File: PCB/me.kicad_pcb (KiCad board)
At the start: 2 copper layers, 166.7 x 154.5 mm, 14 parts, among them M1 Motor_DC, Q1 AO3400A, SW1 SW_Push, SW2 SW_Push, SW3 SW_Push, SW4 SW_Push, SW5 SW_Push, SW6 SW_Push, U1 XIAO-RP2040-DIP

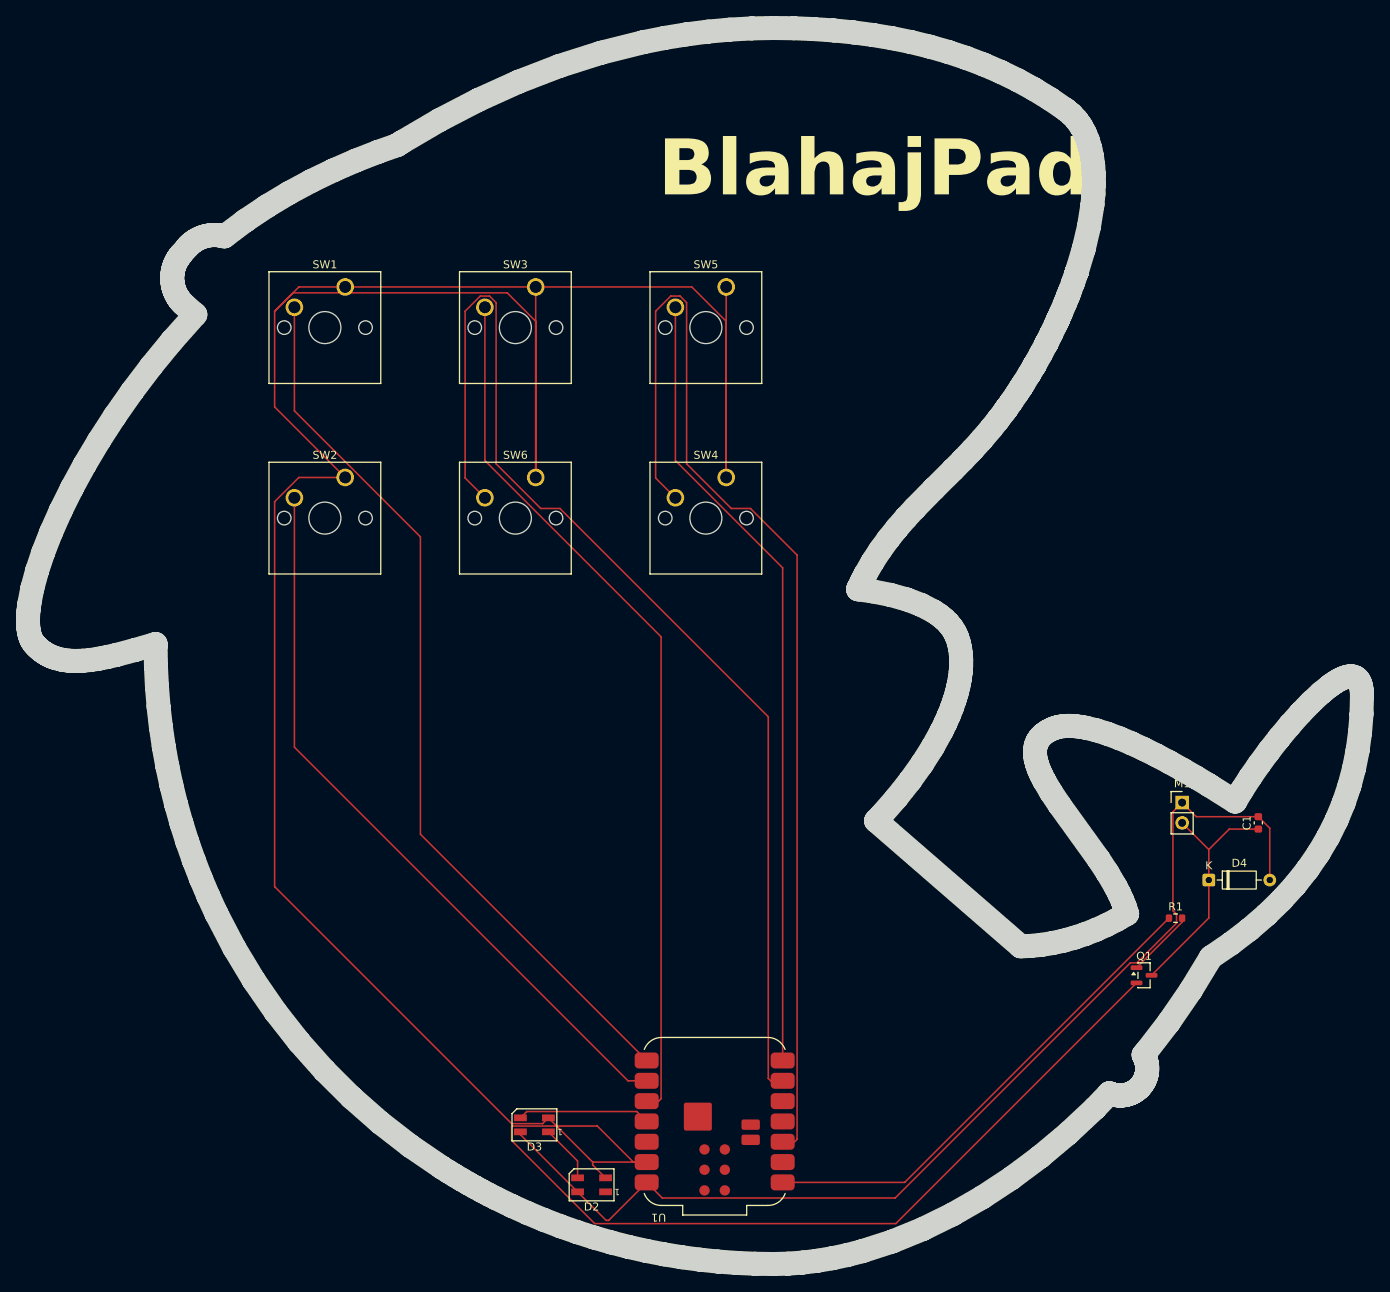
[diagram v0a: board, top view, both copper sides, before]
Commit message: please
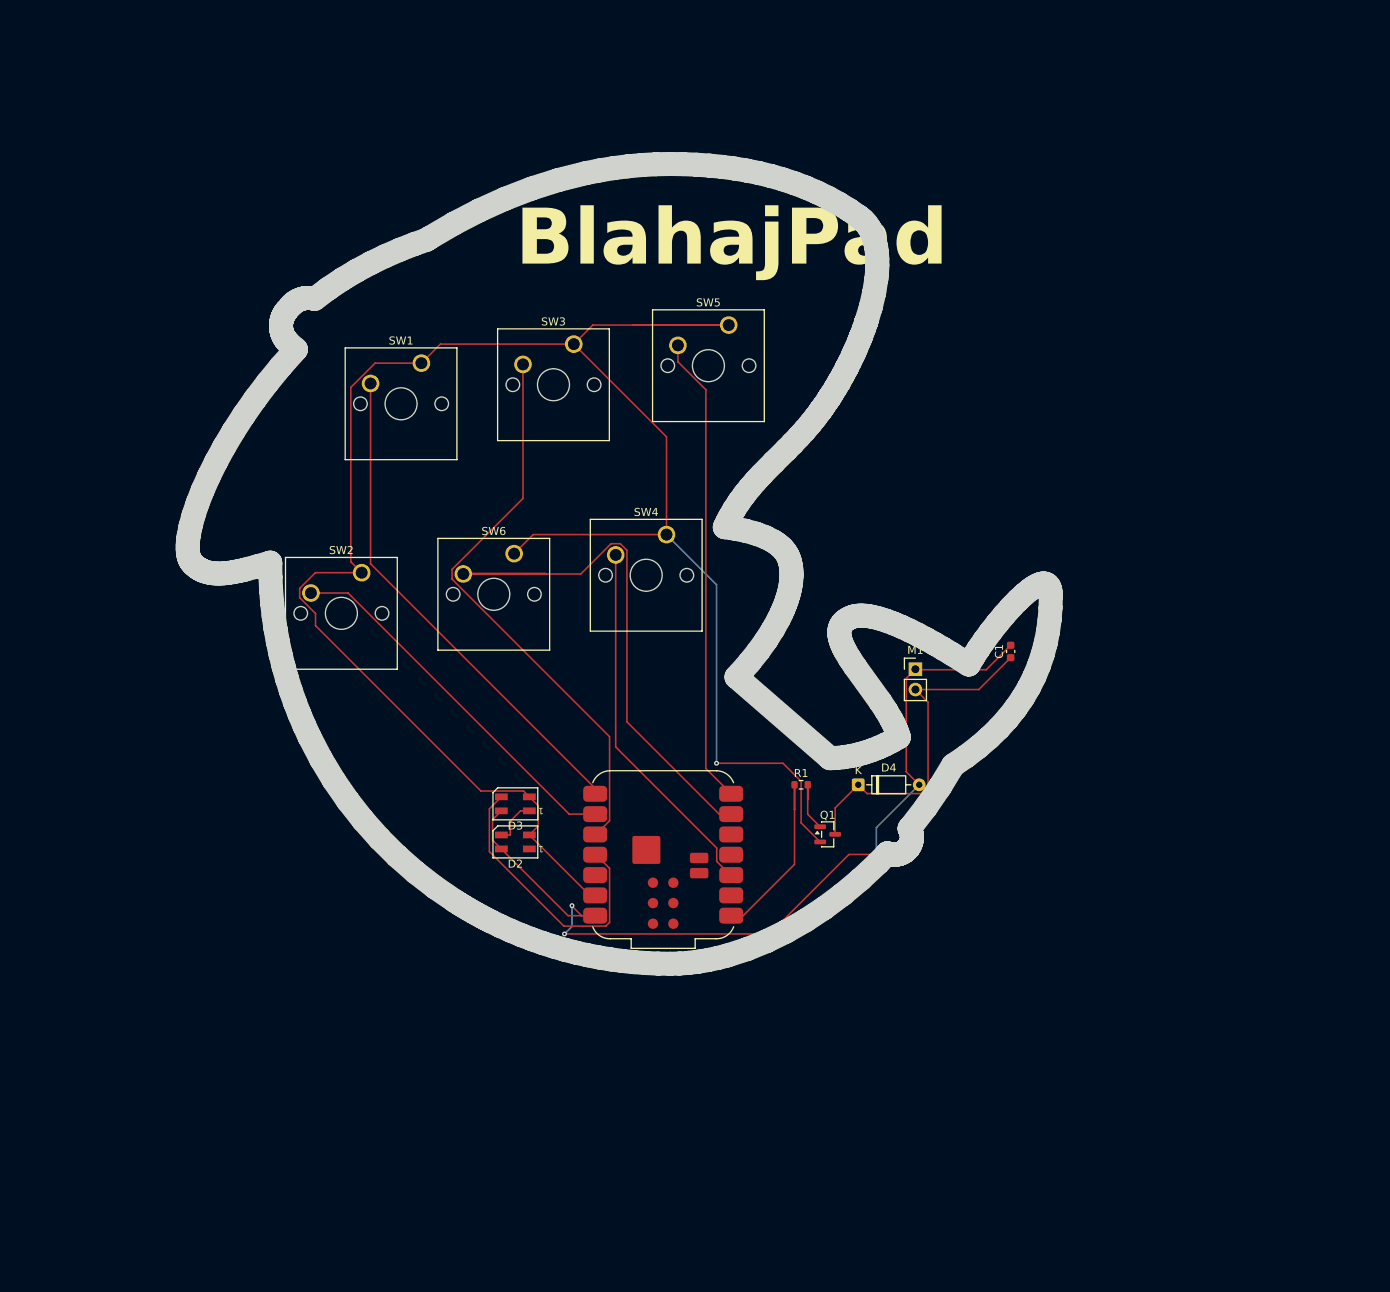
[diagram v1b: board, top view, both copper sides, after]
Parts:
- moved R1 49.7 mm to (173.8, 126.2)
- moved D4 45.4 mm to (181.0, 126.2)
- moved D2 43.9 mm to (138.1, 133.3)
- moved Q1 43.3 mm to (177.2, 132.4)
- moved D3 40.2 mm to (138.1, 128.6)
- moved C1 37.7 mm to (200.0, 109.5)
- moved M1 37.3 mm to (188.1, 111.8)
- moved U1 34.0 mm to (156.6, 134.9)
- moved SW1 13.5 mm to (126.4, 73.5)
- moved SW2 12.1 mm to (118.9, 99.7)
- moved SW4 10.3 mm to (157.0, 94.9)
- moved SW6 9.90 mm to (138.0, 97.3)
- moved SW3 8.59 mm to (145.4, 71.1)
- moved SW5 4.77 mm to (164.8, 68.7)
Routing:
- net GND: track 443.3 -> 252.7 mm, vias 0 -> 1
- net Net-(U1-GPIO28/ADC2/A2): track 143.0 -> 47.6 mm
- net Net-(U1-GPIO7/SCL): track 143.7 -> 72.9 mm
- net Net-(U1-GPIO1/RX): track 112.4 -> 63.5 mm
- net Net-(U1-GPIO2/SCK): track 92.5 -> 47.0 mm
- net Net-(U1-GPIO0/TX): track 99.7 -> 60.8 mm
- net Net-(U1-GPIO26/ADC0/A0): track 62.0 -> 23.6 mm
- net Net-(U1-GPIO4/MISO): track 110.0 -> 72.1 mm
- net +5V: track 138.3 -> 109.4 mm, vias 0 -> 3
- net Net-(D3-DIN): track 16.6 -> 35.8 mm
- net Net-(D4-K): track 30.6 -> 45.1 mm
- net Net-(D2-DIN): track 7.26 -> 5.75 mm
- net Net-(Q1-G): track 8.55 -> 7.73 mm
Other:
- board size 166.7 x 154.5 mm -> 107.9 x 100 mm
